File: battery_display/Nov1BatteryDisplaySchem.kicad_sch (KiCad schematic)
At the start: 21 parts, among them Q1 ZXM61N03F, U1 E2206KS0E1, U2 NCP1117LPST33T3G

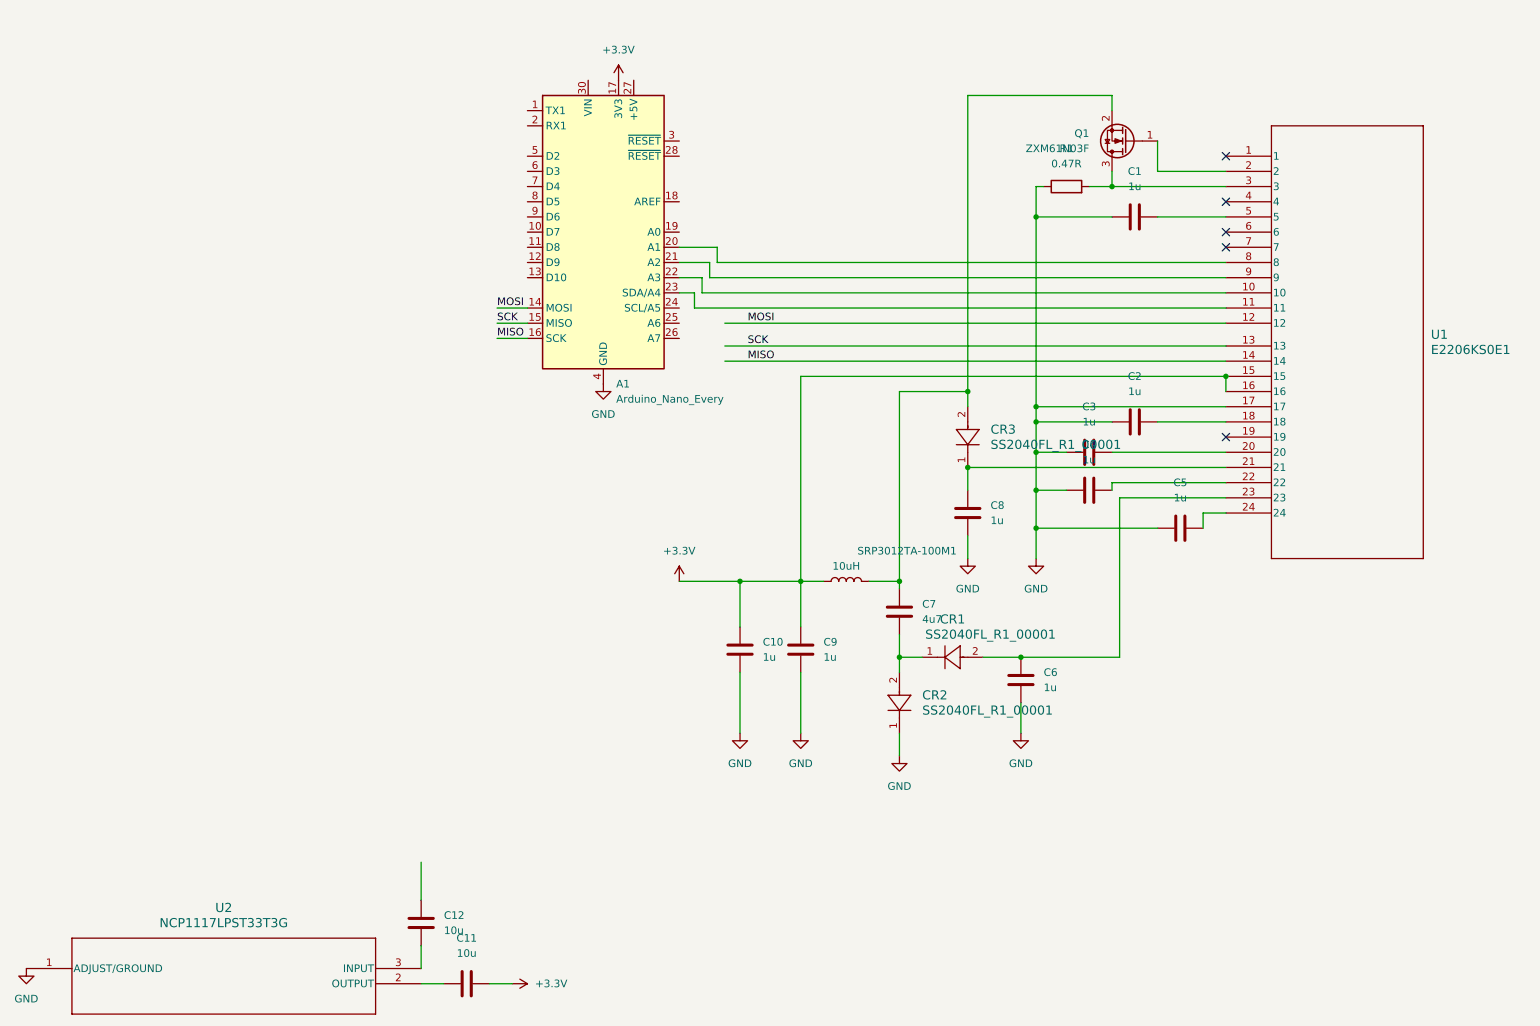
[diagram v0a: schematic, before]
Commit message: Nov8 update
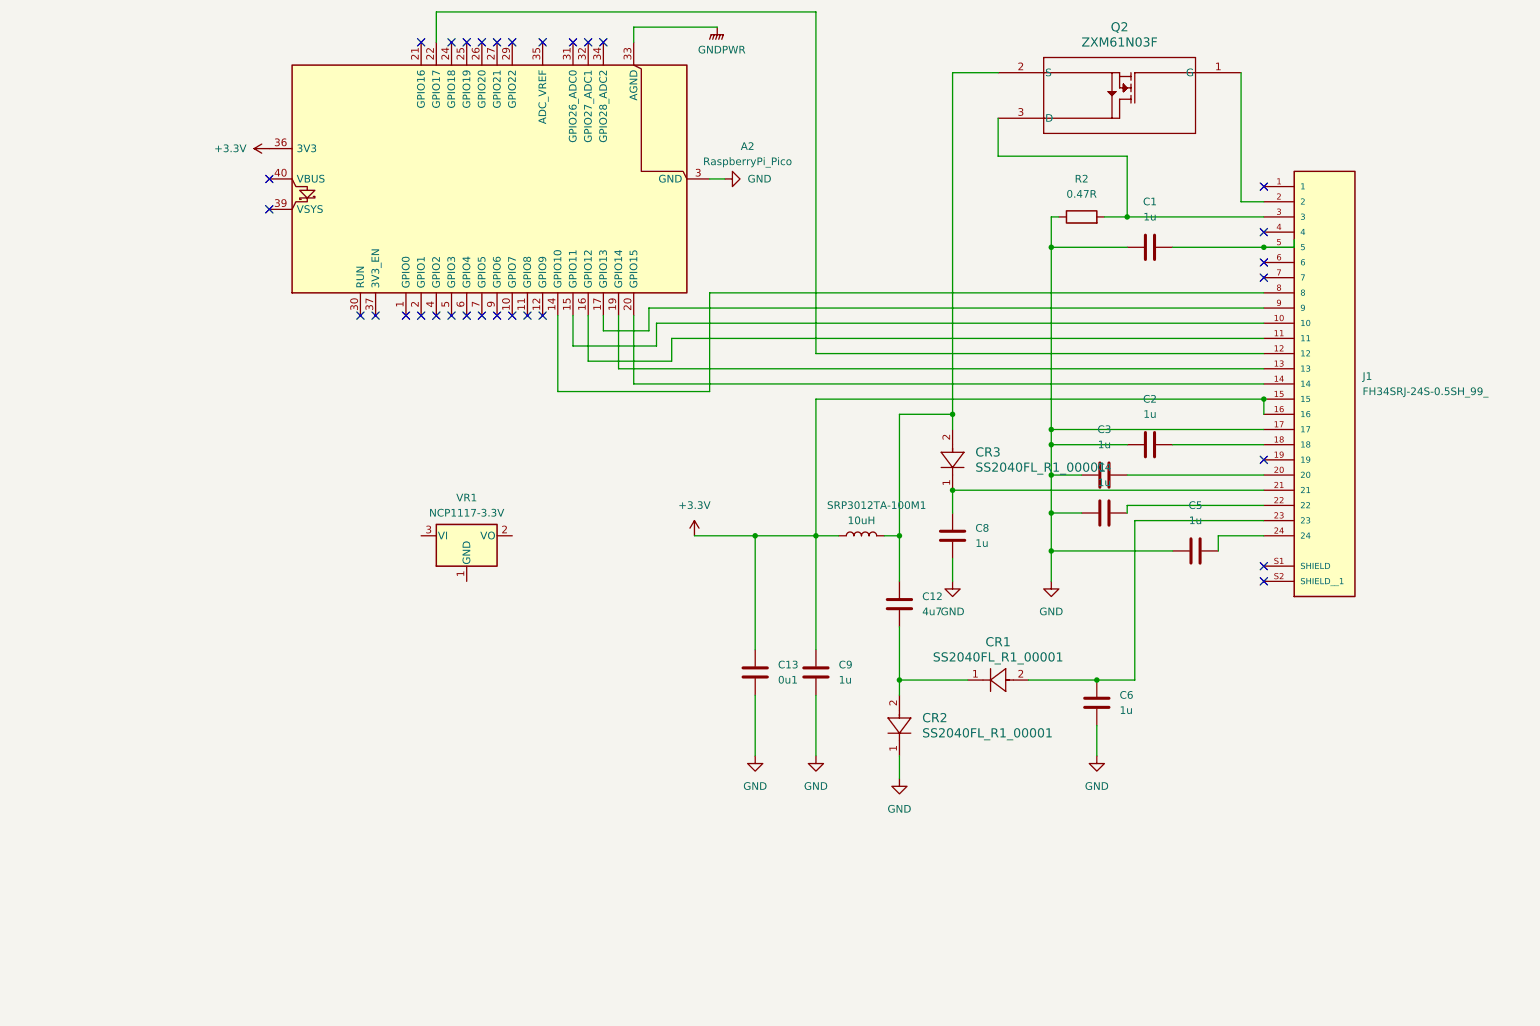
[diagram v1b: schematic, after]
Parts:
- removed A1: Arduino_Nano_Every, Module:Arduino_Nano, symbol MCU_Module:Arduino_Nano_Every
- removed C10: 1u, rsx_capacitors:C_0805_2012Metric, symbol rsx_Capacitors:1u
- removed C11, C12: 10u, rsx_capacitors:C_0805_2012Metric, symbol rsx_Capacitors:10u
- removed C7: 4u7, rsx_capacitors:C_0805_2012Metric, symbol rsx_Capacitors:4u7
- removed Q1: ZXM61N03F, Package_TO_SOT_SMD:SOT-23, symbol Transistor_FET:ZXM61N03F
- removed R1: 0.47R, rsx_resistors:R_1206_3216Metric, symbol rsx_Resistors:0.47R
- removed U1: E2206KS0E1, symbol rsx_misc:Graphic Display
- removed U2: NCP1117LPST33T3G, SOT223-3_ONS, symbol NCP1117:NCP1117LPST33T3G
- added A2: RaspberryPi_Pico, Module:RaspberryPi_Pico_Common_Unspecified, symbol MCU_Module:RaspberryPi_Pico
- added C12: 4u7, rsx_capacitors:C_0805_2012Metric, symbol rsx_Capacitors:4u7
- added C13: 0u1, rsx_capacitors:C_0603_1608Metric, symbol rsx_Capacitors:0u1
- added J1: FH34SRJ-24S-0.5SH_99_, rsx_headers_communications:HRS_FH34SRJ-24S-0.5SH_99_, symbol rsx_Header_communication:FH34SRJ-24S-0.5SH_99_
- added Q2: ZXM61N03F, rsx_packages_TO_SOT:SOT-23, symbol rsx_Transistors:ZXM61N03F
- added R2: 0.47R, rsx_resistors:R_1206_3216Metric, symbol rsx_Resistors:0.47R
- added VR1: NCP1117-3.3V, rsx_packages_TO_SOT:SOT-223-3_TabPin2, symbol rsx_voltage_regulation:NCP1117-3.3V
- CR1, CR2, CR3: footprint CR_R1_00001_PNJ -> Diode_SMD:Nexperia_CFP3_SOD-123W; DPN (none) -> 3757-SS2040FL_R1_00001CT-ND; MPN (none) -> SS2040FL_R1_00001; Manufacturer (none) -> Panjit International Inc.
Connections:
- net +3.3V: now also A2.36 (3V3), C13.1, J1.15, J1.16
- net GND: now also A2.13 (GND), A2.18 (GND), A2.23 (GND), A2.28 (GND), A2.3 (GND), A2.38 (GND), A2.8 (GND), C13.2, J1.17, R2.1
- net at C1.2: now also J1.5
- net at C5.1: now also J1.24
- net at C4.2: now also J1.22
- net at C2.2: now also J1.18
- net at C3.2: now also J1.20
- net at C8.1, CR3.1: now also J1.21
- net at C6.1, CR1.2: now also J1.23
- net at CR3.2, SRP3012TA-100M1.2: now also C12.1, Q2.2 (S)
- net at CR1.1, CR2.2: now also C12.2
- new net: J1.3, Q2.3 (D), R2.2
- new net: A2.15 (GPIO11), J1.10
- new net: A2.16 (GPIO12), J1.11
- new net: A2.22 (GPIO17), J1.12
- new net: A2.19 (GPIO14), J1.13
- new net: A2.20 (GPIO15), J1.14
- new net: J1.2, Q2.1 (G)
- new net: A2.14 (GPIO10), J1.8
- new net: A2.17 (GPIO13), J1.9
- new net GNDPWR: A2.33 (AGND)
- no-connect marks 5 -> 31
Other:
- moved on the sheet: C1, C2, C3, C4, C5, C6, C8, C9, SRP3012TA-100M1
